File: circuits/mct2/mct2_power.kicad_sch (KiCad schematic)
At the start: 275 parts, among them J3 USB_C_Receptacle, J4 USB_C_Receptacle, U4 TPD4USB_EXT30, U5 TPD4USB_EXT30, U6 TPD4USB_EXT30, U7 TPD4USB_EXT30, U9 TPD6S300A

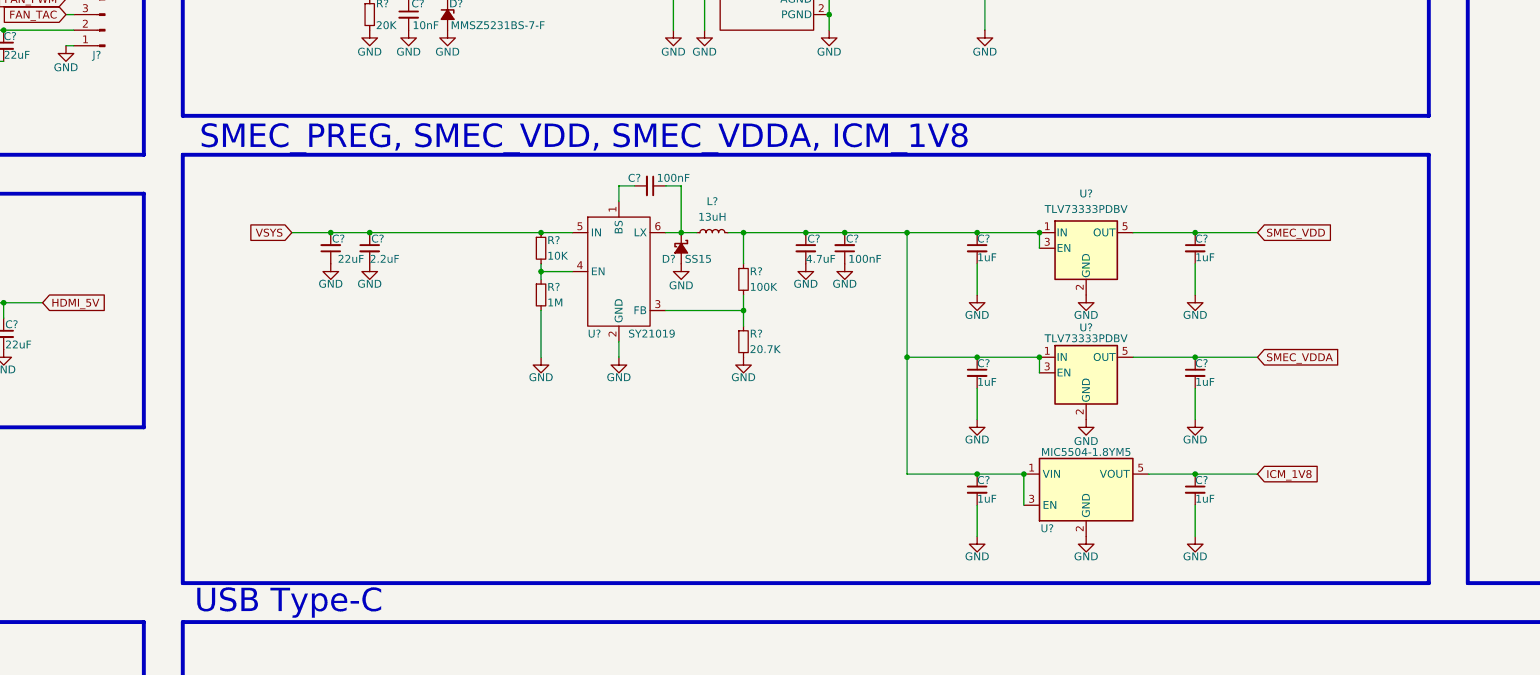
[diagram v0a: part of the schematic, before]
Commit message: Sep 12, 2024 2
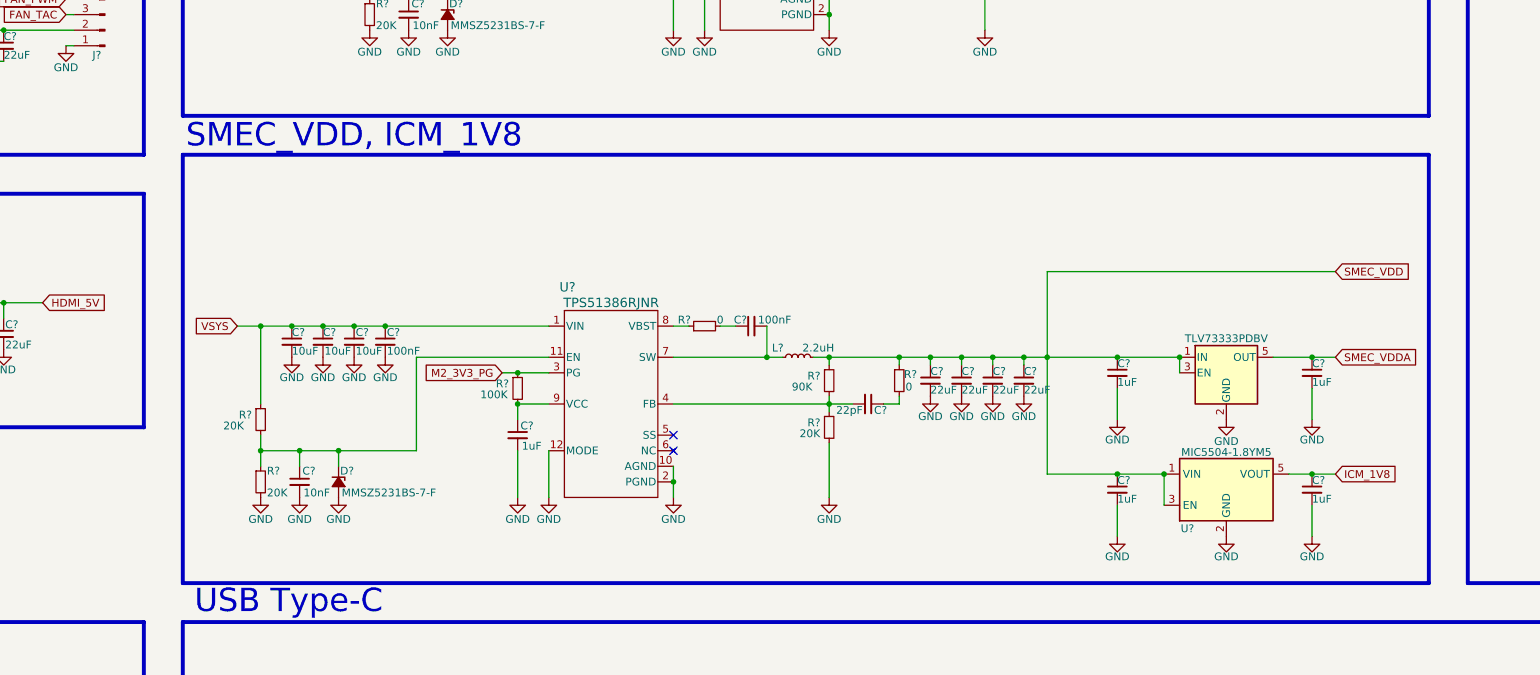
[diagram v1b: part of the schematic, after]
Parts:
- removed C? (x2): 100nF, symbol Device:C_Small
- removed C?: 22uF, symbol Device:C_Small
- removed C?: 2.2uF, symbol Device:C_Small
- removed C? (x2): 1uF, symbol Device:C_Small
- removed C?: 4.7uF, symbol Device:C_Small
- removed D?: SS15, Diode_SMD:D_SMA, symbol Device:D_Schottky_Small_Filled
- removed L?: 13uH, symbol Device:L_Small
- removed R?: 20.7K, symbol Device:R_Small
- removed R?: 10K, symbol Device:R_Small
- removed R?: 1M, symbol Device:R_Small
- removed R?: 100K, symbol Device:R_Small
- removed U?: TLV73333PDBV, Package_TO_SOT_SMD:SOT-23-5, symbol Regulator_Linear:TLV73333PDBV
- removed U?: SY21019, Package_TO_SOT_SMD:SOT-23-6, symbol mediacow:SY21019
- added C? (x3): 10uF, symbol Device:C_Small
- added C? (x4): 22uF, symbol Device:C_Small
- added C? (x2): 100nF, symbol Device:C_Small
- added C?: 1uF, symbol Device:C_Small
- added C?: 22pF, symbol Device:C_Small
- added C?: 10nF, symbol Device:C_Small
- added D?: MMSZ5231BS-7-F, Diode_SMD:D_SOD-323, symbol Device:D_Zener_Small_Filled
- added L?: 2.2uH, symbol Device:L_Small
- added R?: 90K, symbol Device:R_Small
- added R? (x3): 20K, symbol Device:R_Small
- added R?: 100K, symbol Device:R_Small
- added R? (x2): 0, symbol Device:R_Small
- added U?: TPS51386RJNR, VQFN-HR12_RJN_TEX, symbol mediacow:TPS51386RJNR
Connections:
- net GND: now also C?.2, C?.2, C?.2, C?.2, C?.2, C?.2, C?.2, C?.2, C?.2, C?.2, D?.2 (A), R?.2, R?.2, U?.10 (AGND), U?.12 (MODE), U?.2 (PGND)
- net M2_3V3_PG: now also R?.1, U?.3 (PG)
- net SMEC_VDD: now also C?.1, C?.1, U?.1 (IN), U?.1 (VIN), U?.3 (EN), U?.3 (EN), C?.1, C?.1, C?.1, C?.1, L?.2, R?.1, R?.1
- net VSYS: now also C?.1, C?.1, C?.1, C?.1, R?.1, U?.1 (VIN)
- new net: C?.2, R?.1, R?.2, U?.4 (FB)
- new net: C?.1, R?.2, U?.9 (VCC)
- new net: R?.1, U?.8 (VBST)
- new net: C?.1, R?.2 (x2)
- new net: C?.2, L?.1, U?.7 (SW)
- new net: C?.1, D?.1 (K), R?.1, R?.2, U?.11 (EN)
- no-connect marks 23 -> 25
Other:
- note added: "SMEC_VDD, ICM_1V8"
- note removed: "SMEC_PREG, SMEC_VDD, SMEC_VDDA, ICM_1V8"
- moved on the sheet: C?, U?
